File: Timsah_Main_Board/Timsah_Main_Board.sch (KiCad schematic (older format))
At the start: 1 part

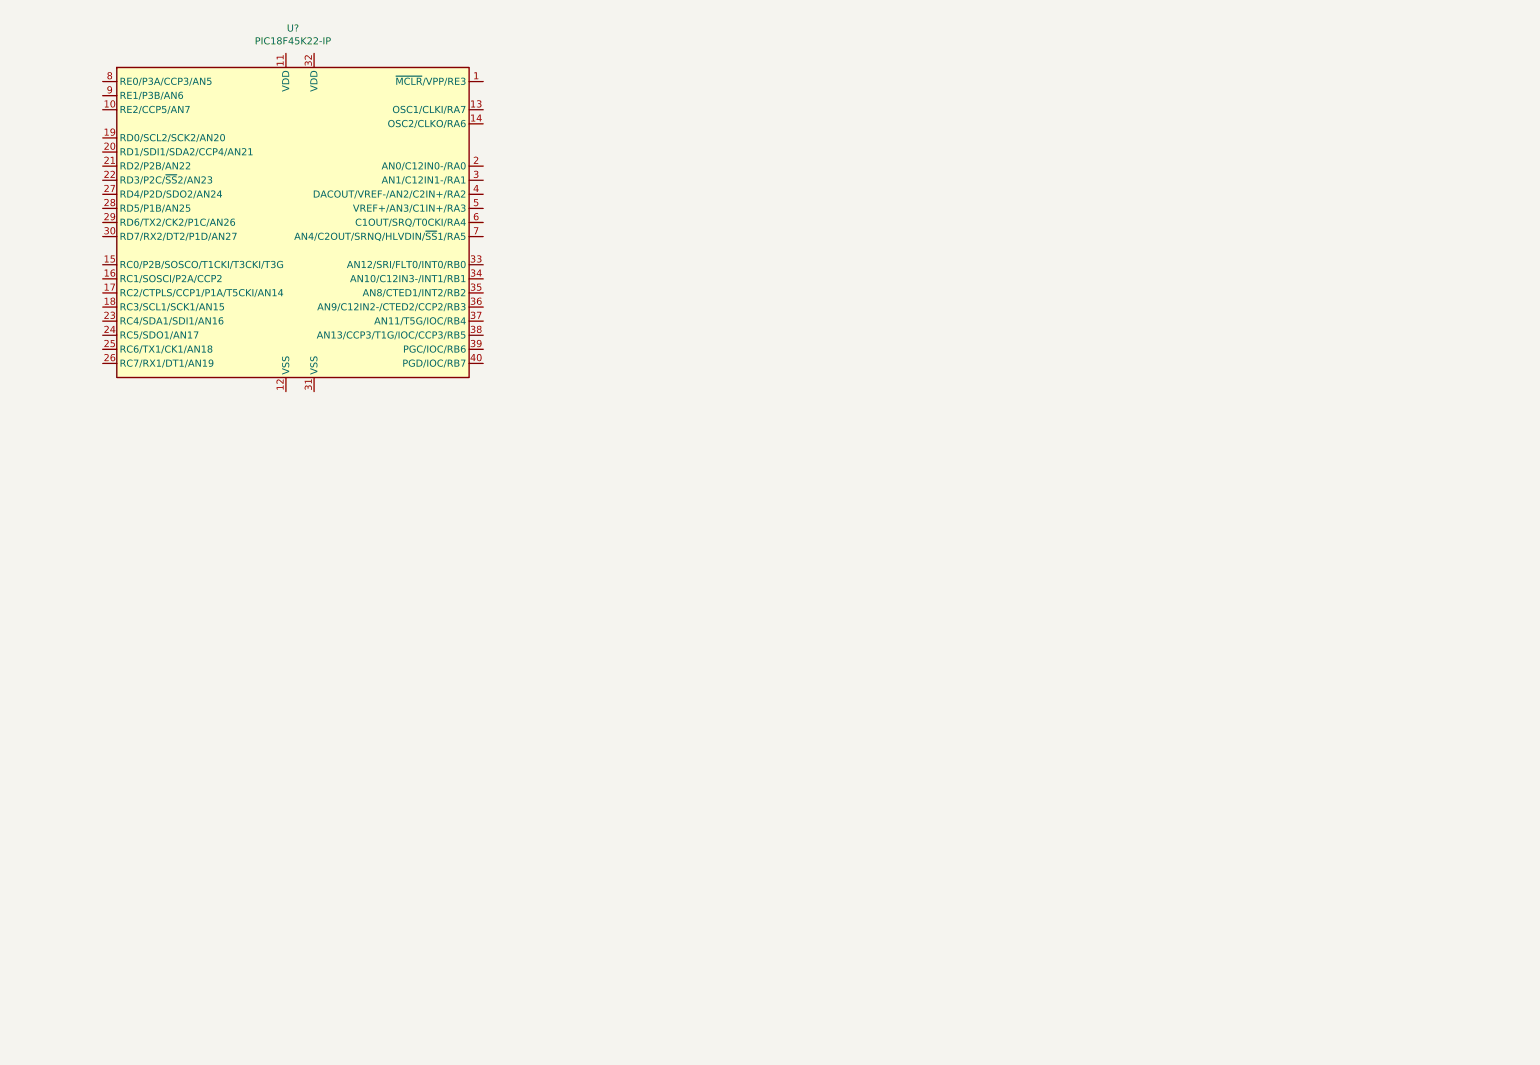
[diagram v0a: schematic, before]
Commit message: Initialize Schematic
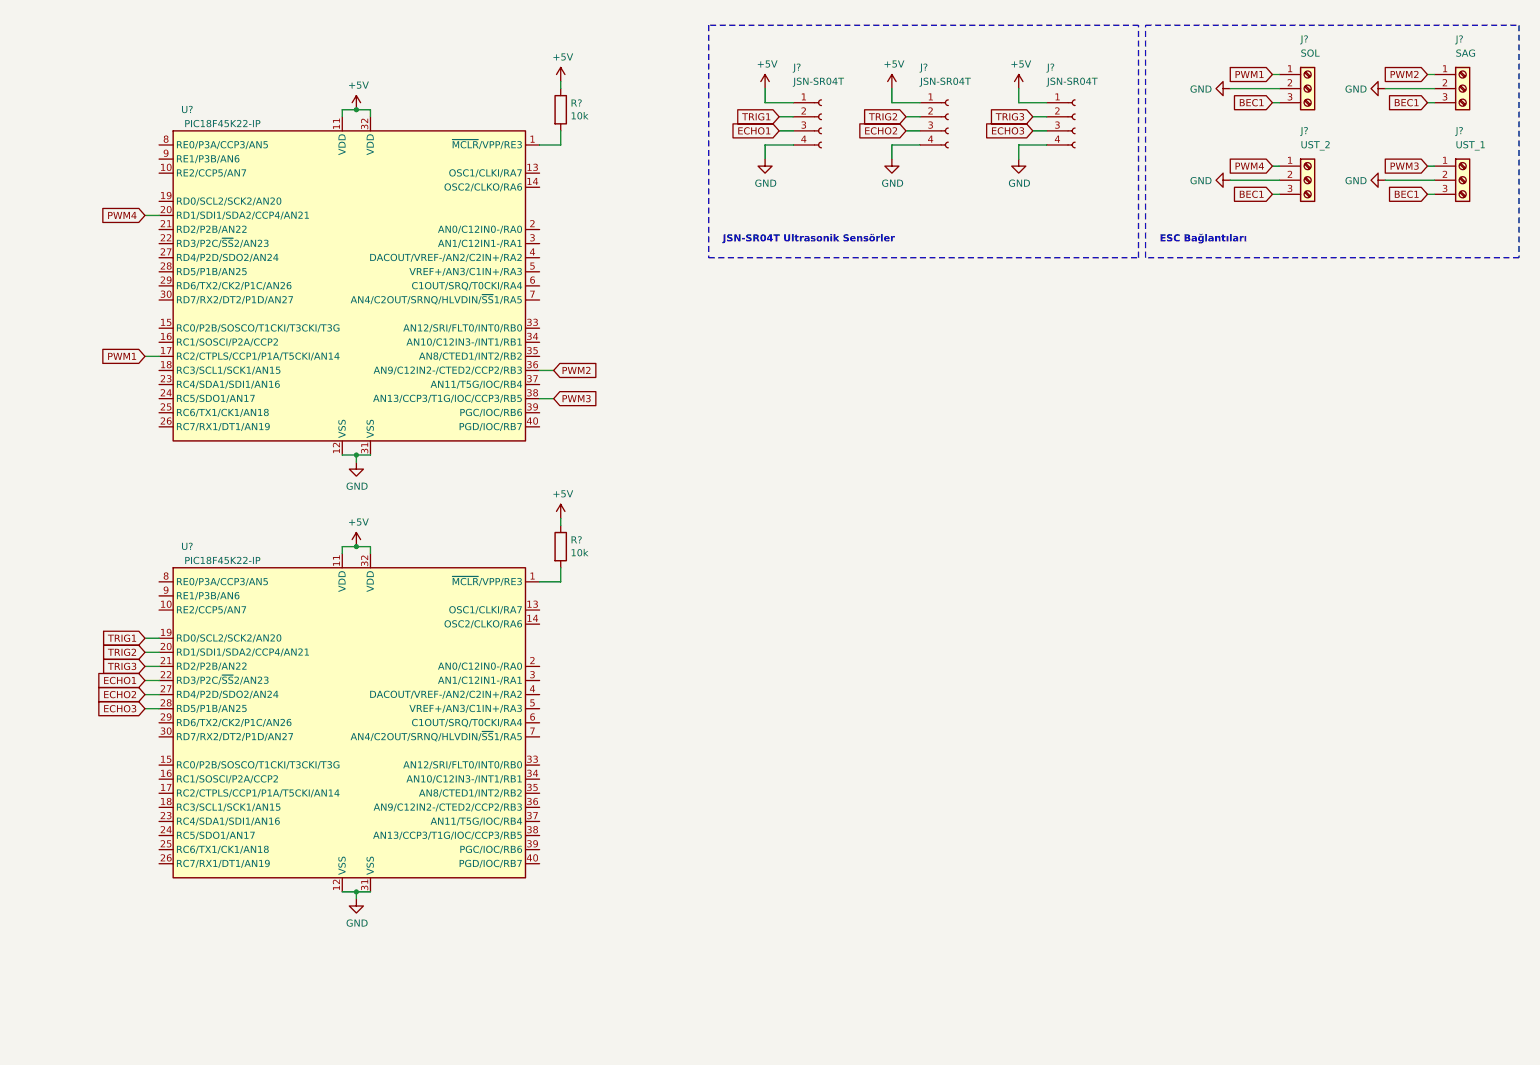
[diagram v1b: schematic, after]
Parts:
- added J?: SAG, symbol Connector:Screw_Terminal_01x03
- added J?: SOL, symbol Connector:Screw_Terminal_01x03
- added J?: UST_1, symbol Connector:Screw_Terminal_01x03
- added J?: UST_2, symbol Connector:Screw_Terminal_01x03
- added J? (x3): JSN-SR04T, symbol Connector:Conn_01x04_Female
- added R? (x2): 10k, symbol Device:R
- added U?: PIC18F45K22-IP, Package_DIP:DIP-42_W15.24mm_LongPads, symbol Symols:PIC18F45K22-IP
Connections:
- net at U?.1 (~MCLR~/VPP/RE3): now also R?.2
- net +5V: now reaches U?.11 (VDD)
- net +5V: now also U?.32 (VDD), J?.1 (Pin_1), J?.1 (Pin_1), J?.1 (Pin_1), R?.1, R?.1, U?.11 (VDD), U?.32 (VDD)
- net GND: now reaches U?.12 (VSS)
- net GND: now also U?.31 (VSS), J?.2 (Pin_2), J?.2 (Pin_2), J?.2 (Pin_2), J?.2 (Pin_2), J?.4 (Pin_4), J?.4 (Pin_4), J?.4 (Pin_4), U?.12 (VSS), U?.31 (VSS)
- net PWM1: now reaches U?.17 (RC2/CTPLS/CCP1/P1A/T5CKI/AN14)
- net PWM1: now also J?.1 (Pin_1)
- net PWM4: now reaches U?.20 (RD1/SDI1/SDA2/CCP4/AN21)
- net PWM4: now also J?.1 (Pin_1)
- net PWM2: now reaches U?.36 (AN9/C12IN2-/CTED2/CCP2/RB3)
- net PWM2: now also J?.1 (Pin_1)
- net PWM3: now reaches U?.38 (AN13/CCP3/T1G/IOC/CCP3/RB5)
- net PWM3: now also J?.1 (Pin_1)
- new net: R?.2, U?.1 (~MCLR~/VPP/RE3)
- new net BEC1: J?.3 (Pin_3), J?.3 (Pin_3), J?.3 (Pin_3), J?.3 (Pin_3)
- new net ECHO1: J?.3 (Pin_3), U?.22 (RD3/P2C/~SS~2/AN23)
- new net ECHO2: J?.3 (Pin_3), U?.27 (RD4/P2D/SDO2/AN24)
- new net ECHO3: J?.3 (Pin_3), U?.28 (RD5/P1B/AN25)
- new net TRIG1: J?.2 (Pin_2), U?.19 (RD0/SCL2/SCK2/AN20)
- new net TRIG2: J?.2 (Pin_2), U?.20 (RD1/SDI1/SDA2/CCP4/AN21)
- new net TRIG3: J?.2 (Pin_2), U?.21 (RD2/P2B/AN22)
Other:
- note added: "ESC Bağlantıları"
- note added: "JSN-SR04T Ultrasonik Sensörler"
- moved on the sheet: U?

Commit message: Update Main Board.
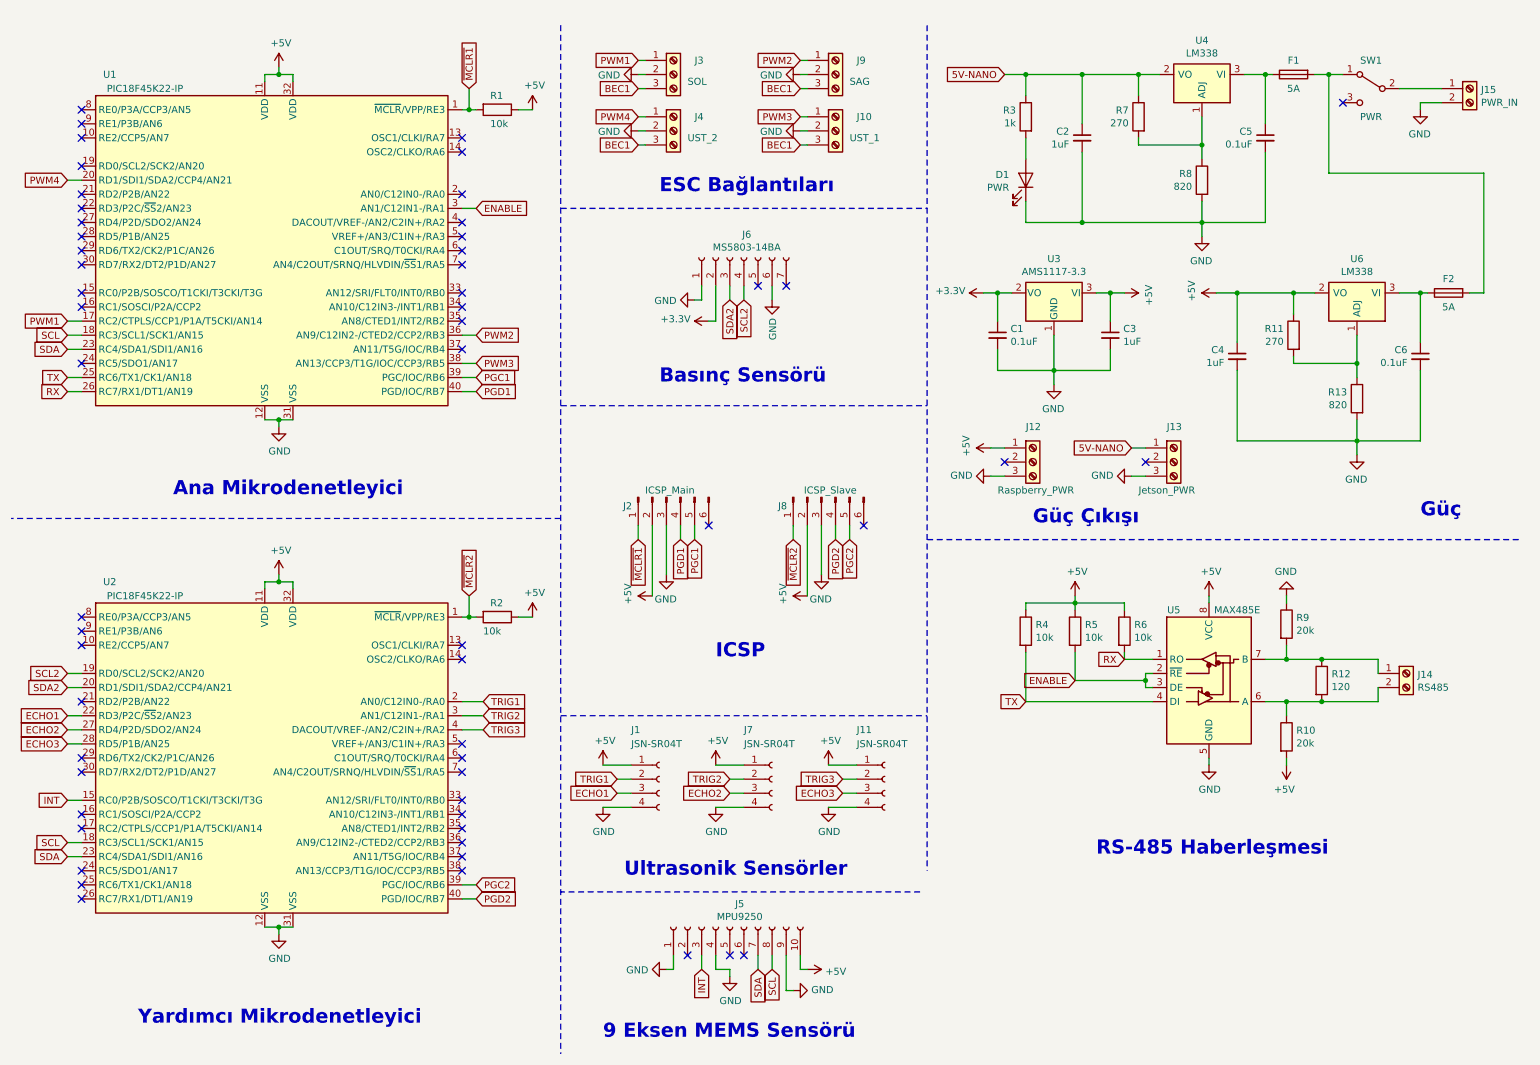
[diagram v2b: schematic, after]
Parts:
- added C1, C5, C6: 0.1uF, symbol Device:C_Small
- added C2, C3, C4: 1uF, symbol Device:C_Small
- added D1: PWR, symbol Device:LED
- added F1, F2: 5A, symbol Device:Fuse
- added J12: Raspberry_PWR, symbol Connector:Screw_Terminal_01x03
- added J13: Jetson_PWR, symbol Connector:Screw_Terminal_01x03
- added J14: RS485, symbol Connector:Screw_Terminal_01x02
- added J15: PWR_IN, symbol Connector:Screw_Terminal_01x02
- added J2: ICSP_Main, symbol Connector:Conn_01x06_Male
- added J5: MPU9250, symbol Connector:Conn_01x10_Female
- added J6: MS5803-14BA, symbol Connector:Conn_01x07_Female
- added J8: ICSP_Slave, symbol Connector:Conn_01x06_Male
- added R10, R9: 20k, symbol Device:R
- added R11, R7: 270, symbol Device:R
- added R12: 120, symbol Device:R
- added R13, R8: 820, symbol Device:R
- added R3: 1k, symbol Device:R
- added R4, R5, R6: 10k, symbol Device:R
- added SW1: PWR, symbol Switch:SW_SPDT
- added U3: AMS1117-3.3, Package_TO_SOT_SMD:SOT-223-3_TabPin2, symbol Regulator_Linear:AMS1117-3.3
- added U4, U6: LM338, Package_TO_SOT_THT:TO-3, symbol Symols:LM338
- added U5: MAX485E, symbol Interface_UART:MAX485E
- gave numbers to parts that had none: 11
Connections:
- net +5V: now also C3.1, C4.1, J12.1 (Pin_1), J2.2 (Pin_2), J5.10 (Pin_10), J8.2 (Pin_2), R10.2, R11.1, R4.1, R5.1, R6.1, U3.3 (VI), U5.8 (VCC), U6.2 (VO)
- net GND: now also C1.2, C2.2, C3.2, C4.2, C5.2, C6.2, D1.1 (K), J12.3 (Pin_3), J13.3 (Pin_3), J15.2 (Pin_2), J2.3 (Pin_3), J5.1 (Pin_1), J5.4 (Pin_4), J5.9 (Pin_9), J6.1 (Pin_1), J6.6 (Pin_6), J8.3 (Pin_3), R13.2, R8.2, R9.1, U3.1 (GND), U5.5 (GND)
- net TRIG1: now also U2.2 (AN0/C12IN0-/RA0); no longer U2.19 (RD0/SCL2/SCK2/AN20)
- net TRIG2: now also U2.3 (AN1/C12IN1-/RA1); no longer U2.20 (RD1/SDI1/SDA2/CCP4/AN21)
- net TRIG3: now also U2.4 (DACOUT/VREF-/AN2/C2IN+/RA2); no longer U2.21 (RD2/P2B/AN22)
- net ~MCLR1: now reaches R1.2, U1.1 (~MCLR~/VPP/RE3)
- net ~MCLR1: now also J2.1 (Pin_1)
- net SCL: now reaches U1.18 (RC3/SCL1/SCK1/AN15)
- net SCL: now also U2.18 (RC3/SCL1/SCK1/AN15), J5.8 (Pin_8)
- net SDA: now reaches U1.23 (RC4/SDA1/SDI1/AN16)
- net SDA: now also U2.23 (RC4/SDA1/SDI1/AN16), J5.7 (Pin_7)
- net TX: now reaches U1.25 (RC6/TX1/CK1/AN18)
- net TX: now also R4.2, U5.4 (DI)
- net RX: now reaches U1.26 (RC7/RX1/DT1/AN19)
- net RX: now also R6.2, U5.1 (RO)
- net ENABLE: now reaches U1.3 (AN1/C12IN1-/RA1)
- net ENABLE: now also R5.2, U5.2 (~RE), U5.3 (DE)
- net PGC1: now reaches U1.39 (PGC/IOC/RB6)
- net PGC1: now also J2.5 (Pin_5)
- net PGD1: now reaches U1.40 (PGD/IOC/RB7)
- net PGD1: now also J2.4 (Pin_4)
- net ~MCLR2: now reaches R2.2, U2.1 (~MCLR~/VPP/RE3)
- net ~MCLR2: now also J8.1 (Pin_1)
- net INT: now reaches U2.15 (RC0/P2B/SOSCO/T1CKI/T3CKI/T3G)
- net INT: now also J5.3 (Pin_3)
- net PGC2: now reaches U2.39 (PGC/IOC/RB6)
- net PGC2: now also J8.5 (Pin_5)
- net PGD2: now reaches U2.40 (PGD/IOC/RB7)
- net PGD2: now also J8.4 (Pin_4)
- new net: R7.2, R8.1, U4.1 (ADJ)
- new net: C5.1, F1.1, U4.3 (VI)
- new net: F1.2, F2.2, SW1.1 (A)
- new net: J15.1 (Pin_1), SW1.2 (B)
- new net: D1.2 (A), R3.2
- new net: R11.2, R13.1, U6.1 (ADJ)
- new net: C6.1, F2.1, U6.3 (VI)
- new net: J14.2 (Pin_2), R10.1, R12.2, U5.6 (A)
- new net: J14.1 (Pin_1), R12.1, R9.2, U5.7 (B)
- new net +3V3: C1.1, J6.2 (Pin_2), U3.2 (VO)
- new net 5V-NANO: C2.1, J13.1 (Pin_1), R3.1, R7.1, U4.2 (VO)
- new net SCL2: J6.4 (Pin_4), U2.19 (RD0/SCL2/SCK2/AN20)
- new net SDA2: J6.3 (Pin_3), U2.20 (RD1/SDI1/SDA2/CCP4/AN21)
- no-connect marks 0 -> 56
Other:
- note added: "9 Eksen MEMS Sensörü"
- note added: "Ana Mikrodenetleyici"
- note added: "Basınç Sensörü"
- note added: "Güç"
- note added: "Güç Çıkışı"
- note added: "ICSP"
- note added: "RS-485 Haberleşmesi"
- note added: "Ultrasonik Sensörler"
- note added: "Yardımcı Mikrodenetleyici"
- note removed: "JSN-SR04T Ultrasonik Sensörler"
- moved on the sheet: J1, J10, J11, J3, J4, J7, J9, R1, R2, U1, U2
